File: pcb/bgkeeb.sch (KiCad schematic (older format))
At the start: 102 parts, among them J1 Pimoroni, SW1 SW_Push, SW11 SW_Push, SW12 SW_Push, SW13 SW_Push, SW14 SW_Push, SW15 SW_Push, SW2 SW_Push, SW21 SW_Push, SW22 SW_Push, SW23 SW_Push, SW24 SW_Push, SW25 SW_Push, SW3 SW_Push, SW34 SW_Push, SW35 SW_Push, SW4 SW_Push, SW41 SW_Push, SW42 RotaryEncoder_Switch, SW5 SW_Push, SW6 SW_Push, SW7 RotaryEncoder_Switch, SW8 SW_Push, U1 ProMicro, U3 TRRS, U4 TRRS

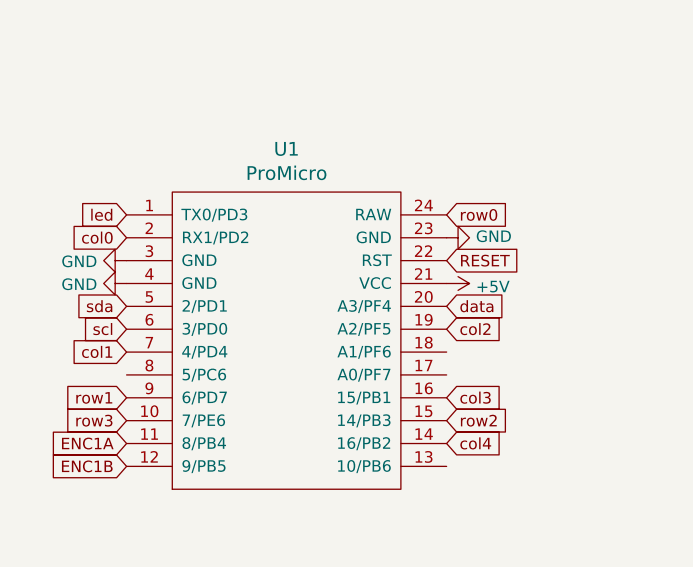
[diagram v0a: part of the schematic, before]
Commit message: fixed a lot of things
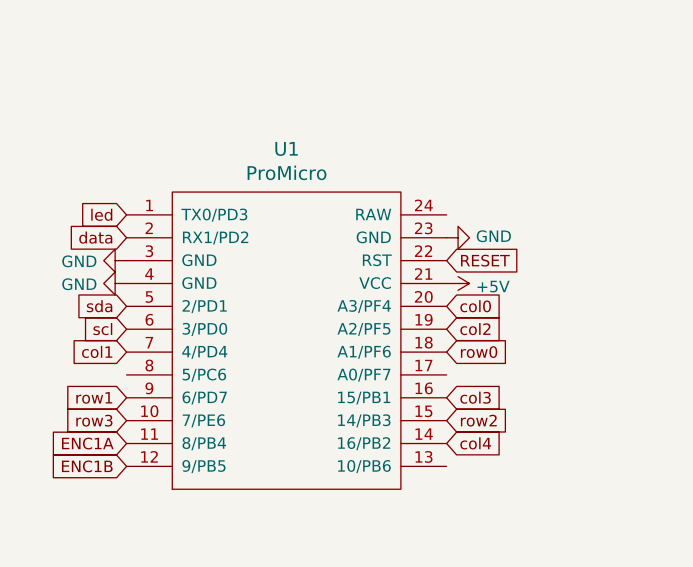
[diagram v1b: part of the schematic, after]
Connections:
- net col0: now also U1.20 (A3/PF4); no longer U1.2 (RX1/PD2)
- net data: now also U1.2 (RX1/PD2); no longer U1.20 (A3/PF4)
- net row0: now also U1.18 (A1/PF6); no longer U1.24 (RAW)
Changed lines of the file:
@@
 Text GLabel 1750 3550 0    50   Input ~ 0
 row3
-Text GLabel 3150 2650 2    50   Input ~ 0
+Text GLabel 3150 3250 2    50   Input ~ 0
 row0
 Text GLabel 1750 3450 0    50   Input ~ 0
@@
 	0    -1   -1   0
 $EndComp
-Text GLabel 1750 2750 0    50   Input ~ 0
+Text GLabel 3150 3050 2    50   Input ~ 0
 col0
 Text GLabel 1750 3250 0    50   Input ~ 0
@@
 Wire Wire Line
 	2300 7750 2150 7750
-Text GLabel 3150 3050 2    50   Input ~ 0
+Text GLabel 1750 2750 0    50   Input ~ 0
 data
 Wire Wire Line
